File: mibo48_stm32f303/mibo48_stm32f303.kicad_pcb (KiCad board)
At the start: 2 copper layers, 57.1 x 21.6 mm, 30 parts, among them J1 Conn_01x02, J2 Conn_01x22, J3 Conn_01x22, J4 USB_B_Micro, J5 Conn_01x04, SW1 Reset, U1 STM32F303CBTx, U2 AMS1117-3.3, Y1 8MHz

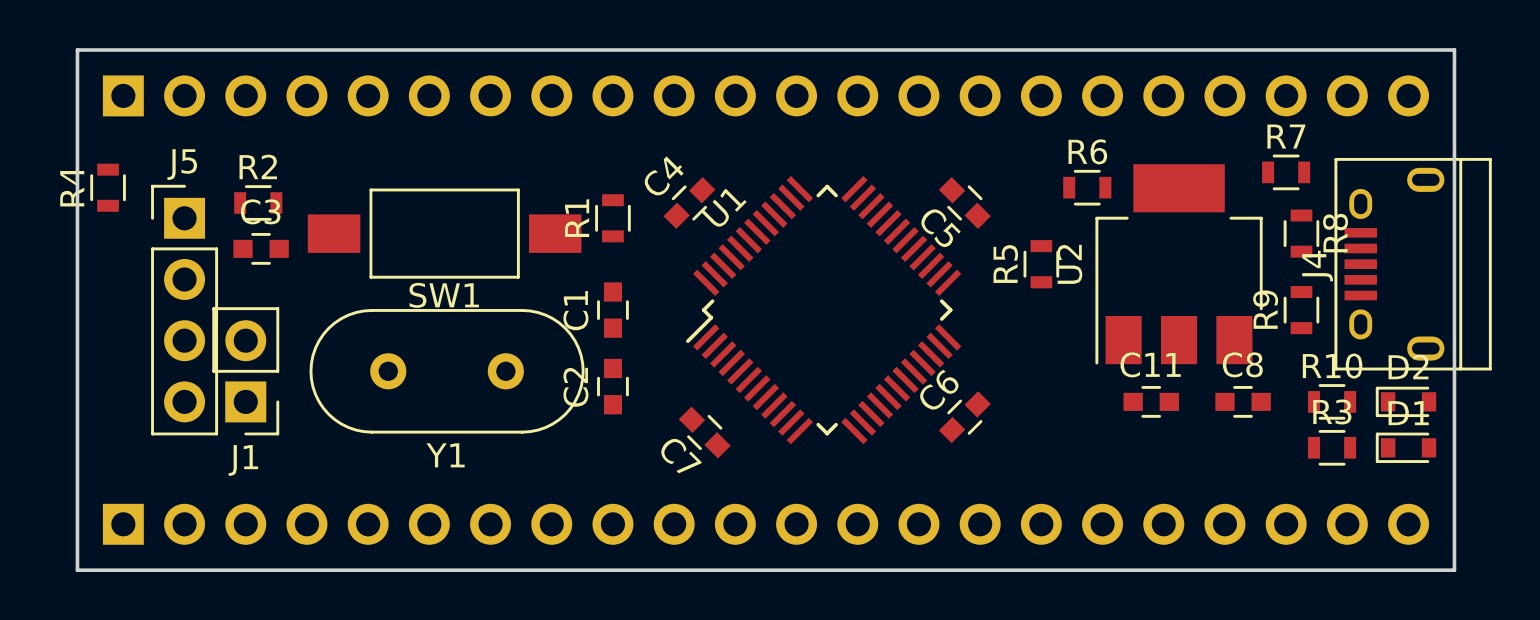
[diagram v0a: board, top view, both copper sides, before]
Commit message: - fully routed, only labelling is missing - kicad 5 project with new libraries and footprints
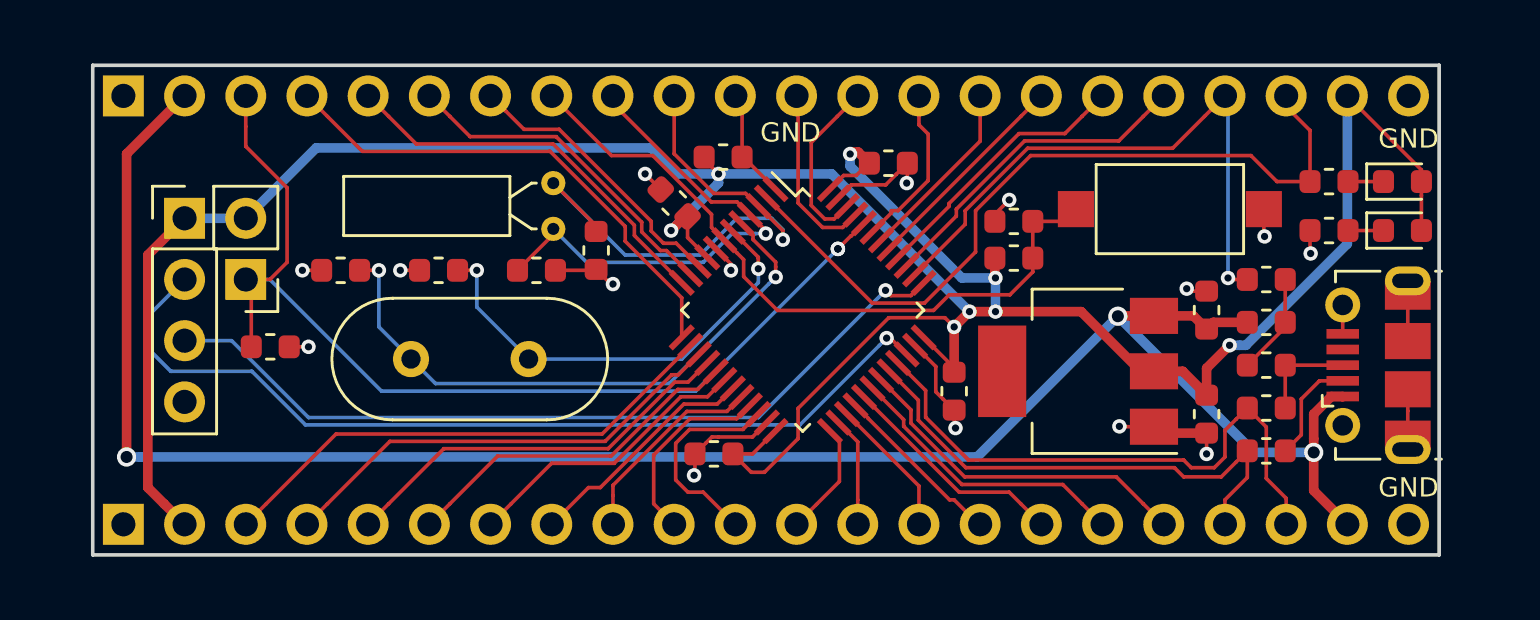
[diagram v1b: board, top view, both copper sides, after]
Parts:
- added C10: 22pF, Capacitor_SMD:C_0603_1608Metric, F.Cu at (146.7, 103.8)
- added C9: 22pF, Capacitor_SMD:C_0603_1608Metric, F.Cu at (149.2, 102.9)
- added Y2: 32.768kHz, Crystal:Crystal_C26-LF_D2.1mm_L6.5mm_Horizontal, F.Cu at (147.4, 100.1)
- C1, C11, C2, C3, C4, C5, C6, C7, C8: footprint Capacitors_SMD:C_0603 -> Capacitor_SMD:C_0603_1608Metric
- D1, D2: footprint Diodes_SMD:D_0603 -> LED_SMD:LED_0603_1608Metric
- J1: footprint Pin_Headers:Pin_Header_Straight_1x02_Pitch2.54mm -> Connector_PinHeader_2.54mm:PinHeader_1x02_P2.54mm_Vertical
- J2, J3: footprint Pin_Headers:Pin_Header_Straight_1x22_Pitch2.54mm -> Connector_PinHeader_2.54mm:PinHeader_1x22_P2.54mm_Vertical
- J4: footprint Connectors:USB_Micro-B -> Connector_USB:USB_Micro-B_Molex-105017-0001
- J5: footprint Pin_Headers:Pin_Header_Straight_1x04_Pitch2.54mm -> Connector_PinHeader_2.54mm:PinHeader_1x04_P2.54mm_Vertical
- R1, R10, R2, R3, R4, R5, R6, R7, R8, R9: footprint Resistors_SMD:R_0603 -> Resistor_SMD:R_0603_1608Metric
- SW1: footprint Buttons_Switches_SMD:SW_SPST_FSMSM -> Button_Switch_SMD:SW_SPST_CK_RS282G05A3
- U1: footprint Housings_QFP:LQFP-48_7x7mm_Pitch0.5mm -> Package_QFP:LQFP-48_7x7mm_P0.5mm
- U2: footprint TO_SOT_Packages_SMD:SOT-223 -> Package_TO_SOT_SMD:SOT-223
- Y1: footprint Crystals:Crystal_HC49-U_Vertical -> Crystal:Crystal_HC49-4H_Vertical
- moved R2 31.4 mm to (166.5, 103.3), turned to 180 degrees
- moved C3 31.3 mm to (166.5, 101.7), turned to 180 degrees
- moved SW1 30.1 mm to (173.0, 101.2), turned to 0 degrees
- moved R4 25.6 mm to (154.4, 99.1), turned to 180 degrees
- moved R1 15.2 mm to (135.6, 106.9), turned to 0 degrees
- moved C1 11.4 mm to (138.6, 103.8), turned to 180 degrees
- moved D1 11.1 mm to (182.6, 100.1)
- moved R3 11.0 mm to (179.6, 100.1)
- moved R5 9.36 mm to (177.0, 104.1), turned to 180 degrees
- moved R6 9.30 mm to (177.0, 105.9)
- moved C2 8.70 mm to (142.6, 103.8), turned to 180 degrees
- moved R7 8.04 mm to (177.0, 107.7), turned to 180 degrees
- moved R8 7.38 mm to (177.0, 109.5), turned to 0 degrees
- moved D2 7.12 mm to (182.6, 102.1)
- moved R10 7.11 mm to (179.6, 102.1)
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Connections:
- D1 pad 1: /LED1 -> Net-(D1-Pad1)
- D1 pad 2: Net-(D1-Pad2) -> +3V3
- D2 pad 1: GND -> Net-(D2-Pad1)
- D2 pad 2: Net-(D2-Pad2) -> +3V3
- J2 pad 10: /PB5 -> /PB10
- J2 pad 11: /PB6 -> /PB11
- J2 pad 12: /PB7 -> /PB12
- J2 pad 13: /PB8 -> /PB13
- J2 pad 14: /PB9 -> /PB14
- J2 pad 15: /PB10 -> /PB15
- J2 pad 16: /PB11 -> /PA8
- J2 pad 17: /PB12 -> /PA9
- J2 pad 18: /PB13 -> /PA10
- J2 pad 19: /PB14 -> /PA11
- J2 pad 20: /PB15 -> /PA12
- J2 pad 3: /BOOT0 -> /PA4
- J2 pad 4: /RESET -> /PA5
- J2 pad 5: /PB0 -> /PA6
- J2 pad 6: /PB1 -> /PA7
- J2 pad 7: /PB2 -> /PB0
- J2 pad 8: /PB3 -> /PB1
- J2 pad 9: /PB4 -> /PB2
- J3 pad 10: /PA6 -> /OSC32_IN
- J3 pad 11: /PA7 -> /VBAT
- J3 pad 12: /PA8 -> /PB8
- J3 pad 13: /PA9 -> /PB9
- J3 pad 14: /PA10 -> /PB7
- J3 pad 15: /PA11 -> /PB6
- J3 pad 16: /PA12 -> /PB5
- J3 pad 17: /PA15 -> /PB4
- J3 pad 18: /LED1 -> /PB3
- J3 pad 19: /OSC32_IN -> /PA15
- J3 pad 20: /OSC32_OUT -> /LED1
- J3 pad 3: /VBAT -> /BOOT0
- J3 pad 4: /PA0 -> /PA3
- J3 pad 5: /PA1 -> /PA2
- J3 pad 6: /PA2 -> /PA1
- J3 pad 7: /PA3 -> /PA0
- J3 pad 8: /PA4 -> /RESET
- J3 pad 9: /PA5 -> /OSC32_OUT
- R10 pad 1: Net-(D2-Pad2) -> GND
- R10 pad 2: +3V3 -> Net-(D2-Pad1)
- R3 pad 1: Net-(D1-Pad2) -> /LED1
- R3 pad 2: +3V3 -> Net-(D1-Pad1)
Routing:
- net +3V3: track 0.00 -> 125.0 mm, vias 0 -> 8
- net /5V: track 0.00 -> 82.4 mm, vias 0 -> 3
- net /BOOT0: track 0.00 -> 43.0 mm, vias 0 -> 2
- net /SWDIO: track 0.00 -> 38.0 mm, vias 0 -> 1
- net /SWDCLK: track 0.00 -> 34.5 mm, vias 0 -> 1
- net GND: track 0.00 -> 33.7 mm, vias 0 -> 15
- net /LED1: track 0.00 -> 32.3 mm
- net /RESET: track 0.00 -> 29.1 mm
- net /OSC_IN: track 0.00 -> 25.2 mm, vias 0 -> 2
- net /PA15: track 0.00 -> 24.7 mm, vias 0 -> 1
- net /PA12: track 0.00 -> 24.1 mm
- net /OSC32_IN: track 0.00 -> 23.4 mm, vias 0 -> 1
- net /PA4: track 0.00 -> 21.5 mm
- net /OSC32_OUT: track 0.00 -> 21.2 mm, vias 0 -> 1
- net /PA3: track 0.00 -> 21.0 mm
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- added copper zone on B.Cu, net GND
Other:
- board size 57.1 x 21.6 mm -> 55.9 x 20.3 mm
- net class Default: clearance 0.2 -> 0.152; trace_width 0.25 -> 0.152; via_dia 0.8 -> 0.6; via_drill 0.4 -> 0.3
- net class power added: clearance 0.152, trace_width 0.4, via_dia 0.8, via_drill 0.5
- rule trace_clearance: 0.2 -> 0.152
- rule trace_min: 0.2 -> 0.152
- rule via_min_size: 0.4 -> 0.6
- board text added: "GND"
